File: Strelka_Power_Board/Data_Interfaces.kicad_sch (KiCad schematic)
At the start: 11 parts

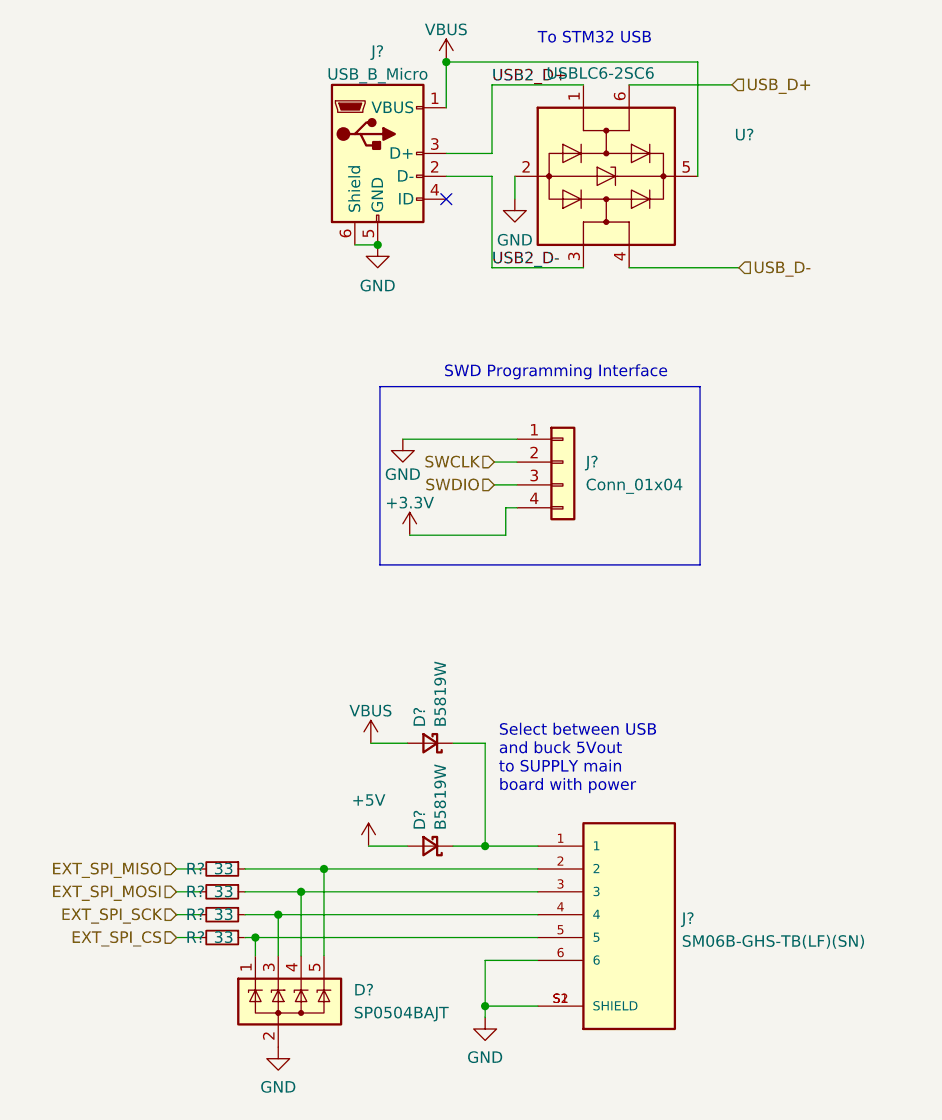
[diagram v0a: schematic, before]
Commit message: Creating BOM
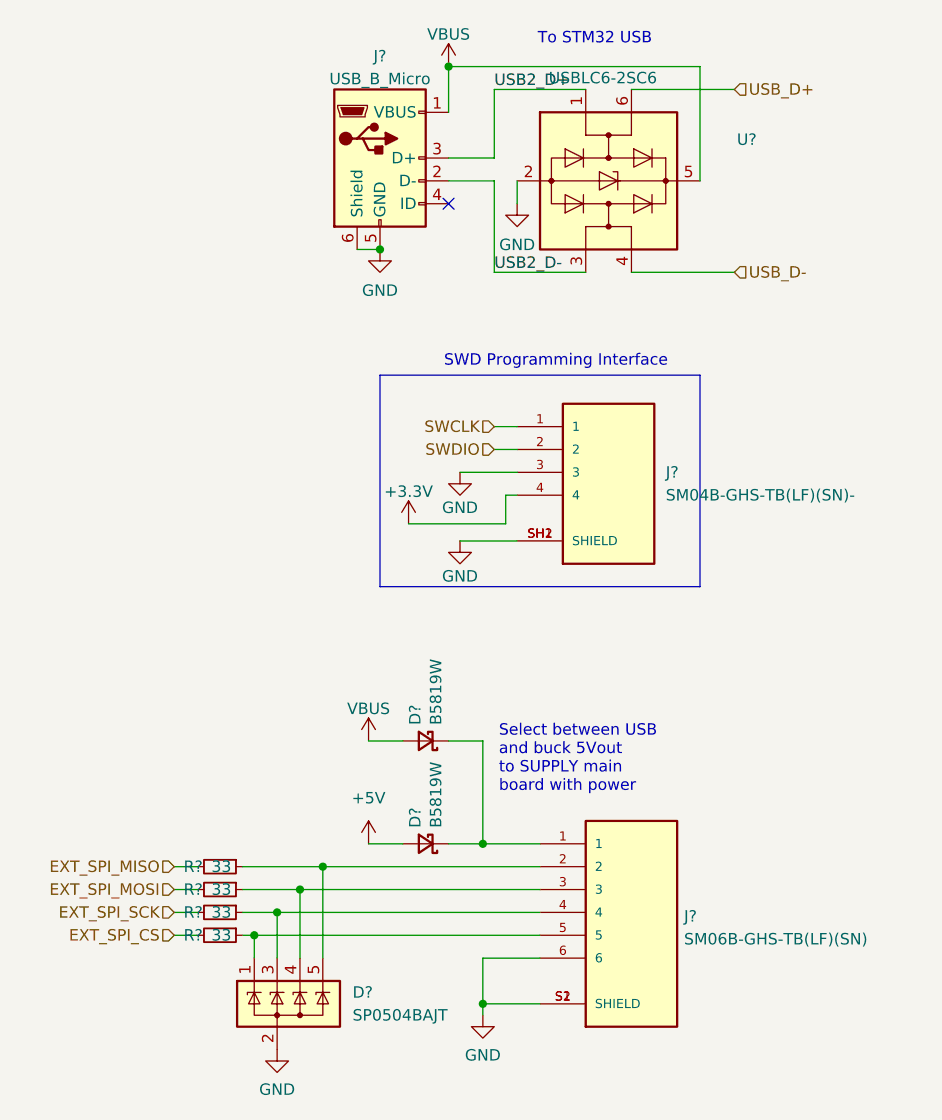
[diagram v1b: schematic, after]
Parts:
- removed J?: Conn_01x04, Connector_PinHeader_2.54mm:PinHeader_1x04_P2.54mm_Horizontal, symbol Connector_Generic:Conn_01x04
- added J?: SM04B-GHS-TB(LF)(SN)-, Footprints:JST_SM04B-GHS-TB(LF)(SN)-, symbol SM04B-GHS-TB_LF__SN_-:SM04B-GHS-TB(LF)(SN)-
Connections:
- net +3V3: now also J?.4
- net GND: now also J?.3, J?.SH1 (SHIELD), J?.SH2 (SHIELD)
- net SWCLK: now also J?.1
- net SWDIO: now also J?.2
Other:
- moved on the sheet: D?, J?, U?
